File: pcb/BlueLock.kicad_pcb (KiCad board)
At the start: 2 copper layers, 47.7 x 22 mm, 47 parts, among them J1 USB_B_Micro, J2 Load, M1 Motor_DC, Q1 Q_NMOS_GSD, Q2 Q_PMOS_GSD, Q3 Q_NMOS_GSD, Q4 Q_PMOS_GSD, Q5 Q_NMOS_GSD, Q6 Q_NMOS_GSD, SW1 SW_Push, U1 TP4057, U2 LN2220, U3 LEM5010, U4 SC662K

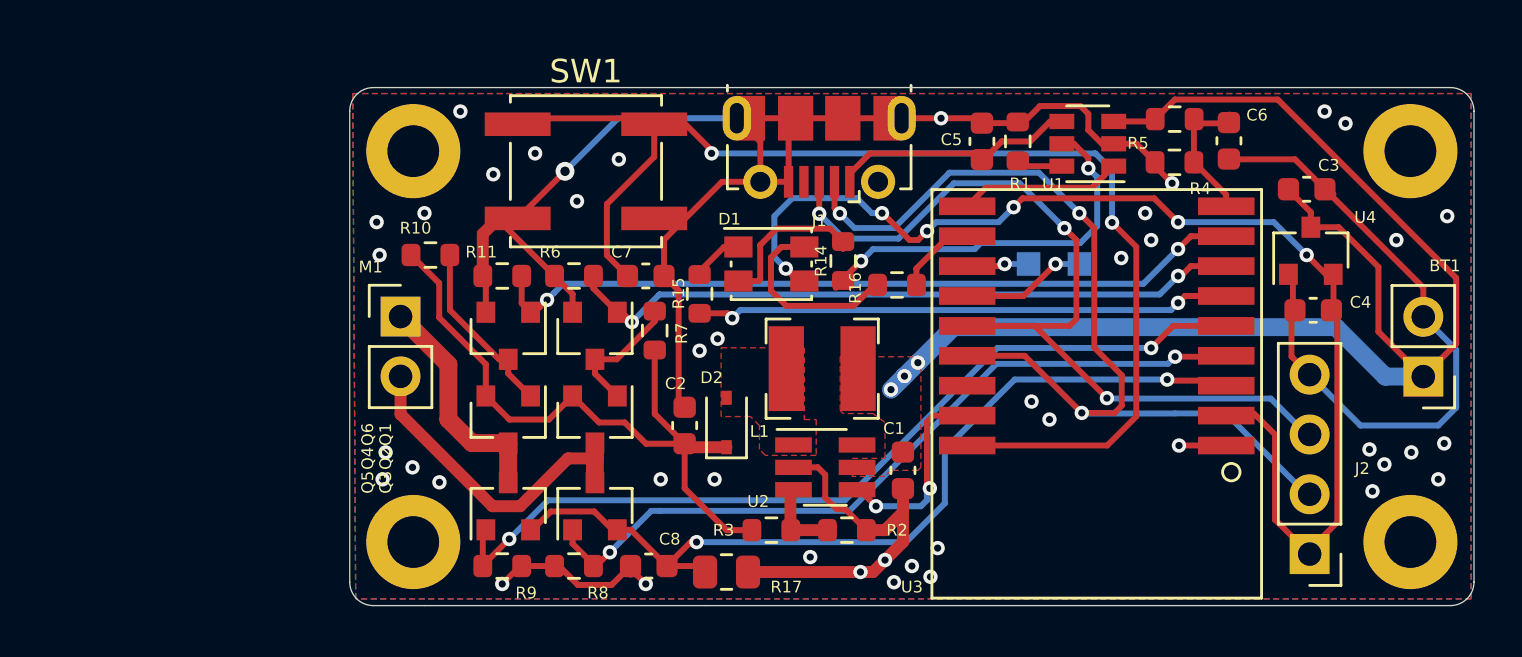
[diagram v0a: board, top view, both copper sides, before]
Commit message: 更新pcb
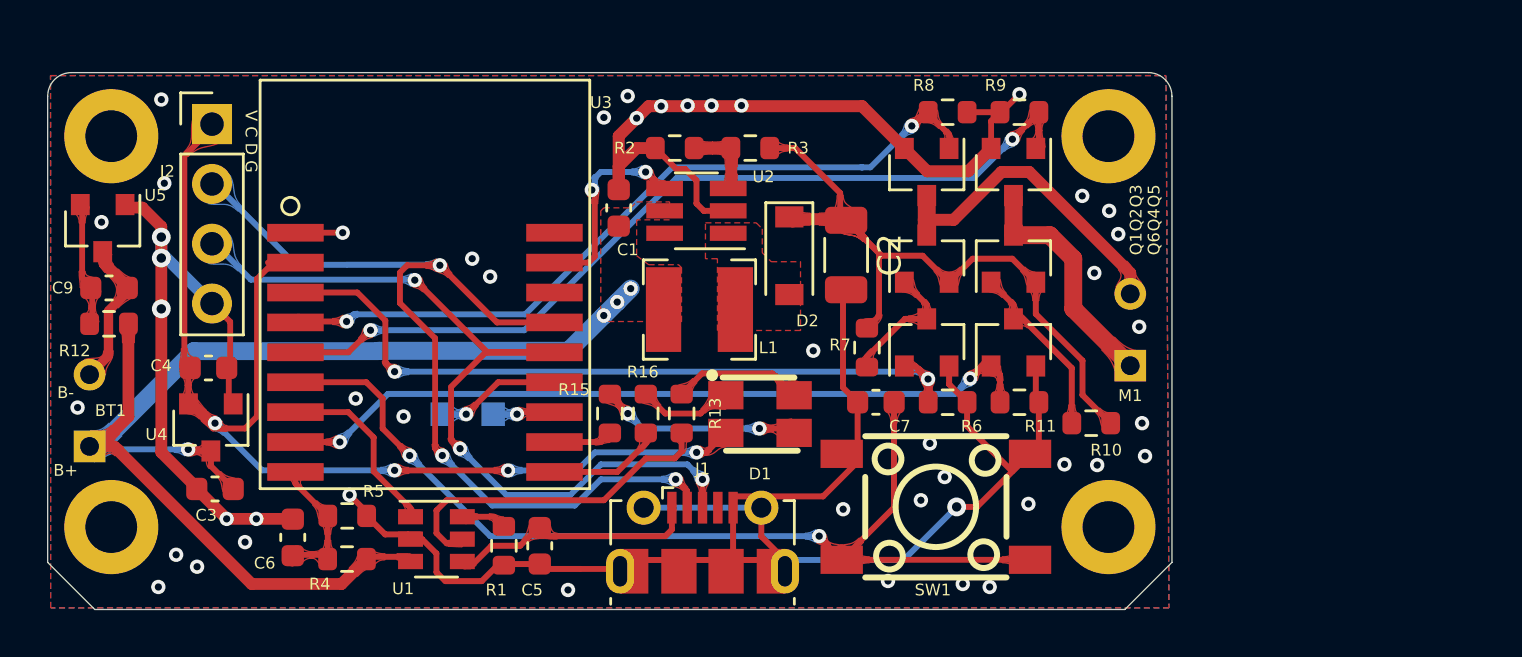
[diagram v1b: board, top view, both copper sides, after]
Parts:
- removed the 0 at (108.7, 70.6)
- removed the 0 at (108.7, 87.2)
- removed the 0 at (66.3, 87.2)
- removed the 0 at (66.3, 70.6)
- removed C8: 10uf, Capacitor_SMD:C_0603_1608Metric
- removed R14: 1k, Resistor_SMD:R_0603_1608Metric
- removed R17: 1R, Resistor_SMD:R_0805_2012Metric
- added 0: R2R4, MyFoot:R2R4, F.Cu at (53.5, 86.6)
- added 0: R2R4, MyFoot:R2R4, F.Cu at (53.5, 70.0)
- added 0: R2R4, MyFoot:R2R4, F.Cu at (95.8, 70.0)
- added 0: R2R4, MyFoot:R2R4, F.Cu at (95.8, 86.6)
- added C9: 0.1uf, Capacitor_SMD:C_0603_1608Metric, F.Cu at (53.4, 76.5)
- added R12: 1K, Resistor_SMD:R_0603_1608Metric, F.Cu at (53.4, 78.0)
- added R13: 1k, Resistor_SMD:R_0603_1608Metric, F.Cu at (77.7, 81.8)
- added U5: XB3306A, Package_TO_SOT_SMD:SOT-23, F.Cu at (53.1, 73.9)
- BT1, M1: footprint Connector_PinHeader_2.54mm:PinHeader_1x02_P2.54mm_Vertical -> Custom:Pin_2_wide
- C2: footprint Capacitor_SMD:C_0603_1608Metric -> Capacitor_SMD:C_1206_3216Metric
- D1: value LED_RBAG -> RGB_1209; footprint LED_SMD:LED_Kingbright_AAA3528ESGCT -> Custom:RGB_1209
- D2: footprint Diode_SMD:D_SOD-323 -> Diode_SMD:D_SOD-123
- R2: value 20k -> 100k
- R3: value 165k -> 750k
- SW1: footprint Button_Switch_SMD:SW_Push_1P1T_NO_CK_KSC6xxJ -> Custom:SW_6x6
- moved BT1 56.7 mm to (52.6, 81.5)
- moved J2 50.1 mm to (57.8, 69.5), turned to 0 degrees
- moved C3 48.1 mm to (57.9, 85.0), turned to 180 degrees
- moved U4 47.3 mm to (57.7, 82.4), turned to 270 degrees
- moved C4 47.0 mm to (57.6, 79.9), turned to 0 degrees
- moved C6 43.2 mm to (61.2, 87.0), turned to 90 degrees
- moved R4 39.8 mm to (63.5, 88.0), turned to 0 degrees
- moved R5 38.2 mm to (63.5, 86.1), turned to 180 degrees
- moved U1 32.4 mm to (67.3, 87.1), turned to 0 degrees
- moved M1 31.0 mm to (96.8, 78.1), turned to 180 degrees
- moved R9 29.2 mm to (92.1, 69.0), turned to 180 degrees
- moved R10 29.0 mm to (95.1, 82.2), turned to 180 degrees
- moved U3 28.9 mm to (66.8, 76.3), turned to 0 degrees
- moved RX1 27.8 mm to (67.6, 81.8), turned to 180 degrees
- moved R1 27.8 mm to (70.2, 87.4), turned to 270 degrees
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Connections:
- BT1 pad 2: GND -> /B-
- Q3 pad 2: /CHK_I -> GND
- Q5 pad 2: /CHK_I -> GND
- R15 pad 1: Net-(D1-Pad1) -> Net-(D1-Pad4)
- R15 pad 2: /LEDR -> /LEDB
- R16 pad 1: Net-(D1-Pad2) -> Net-(D1-Pad1)
- R16 pad 2: /LEDB -> /LEDR
- U1 pad 5: /STDBY -> /LEDG
- U3 pad 10: /CHRG -> /LEDR
- U3 pad 18: /BT -> Net-(U3-Pad18)
- U3 pad 3: /CHK_I -> /H2
- U3 pad 6: /LEDR -> /BT
- U3 pad 7: /H2 -> /CHRG
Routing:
- net /CHK_I: track 37.3 -> 0.00 mm, vias 2 -> 0
- net /LEDR: track 23.0 -> 4.82 mm, vias 2 -> 0
- net /STDBY: track 16.7 -> 0.00 mm, vias 2 -> 0
- net /LEDG: track 0.00 -> 14.4 mm
- net /BT: track 54.9 -> 42.9 mm
- net GND: track 117.6 -> 129.4 mm, vias 44 -> 47
- net /B-: track 0.00 -> 6.29 mm
- net Net-(C9-Pad1): track 0.00 -> 5.14 mm
- net +BATT: track 58.7 -> 54.6 mm, vias 3 -> 4
- net /H2: track 29.0 -> 31.7 mm
- net Net-(D1-Pad2): track 7.87 -> 5.57 mm
- net Net-(D1-Pad1): track 2.55 -> 4.62 mm
- net Net-(D1-Pad4): track 6.77 -> 8.54 mm, vias 0 -> 2
- net /CLK: track 41.4 -> 39.6 mm
- net /VDD: track 50.8 -> 49.4 mm, vias 6 -> 4
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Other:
- board size 47.7 x 22 mm -> 47.7 x 22.8 mm
- board text added: "B+"
- board text added: "B-"
- board text added: "V C D G"
